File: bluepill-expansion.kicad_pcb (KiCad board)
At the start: 2 copper layers, 89.9 x 74.7 mm, 37 parts, among them J1 SENSE_A, J10 ENCODERS, J11 LS2, J12 I/O 3V3, J13 DIGITAL_PWR, J2 SENSE_B, J3 POWER_DC, J4 MOTDC1, J5 MOTDC2, J6 I2C, J7 UART, J8 CAN_BUS, J9 LS1, SW1 LS1, SW2 LS2, U1 BluePill_STM32F103C, U2 L298HN, U3 MCP2551-I-P

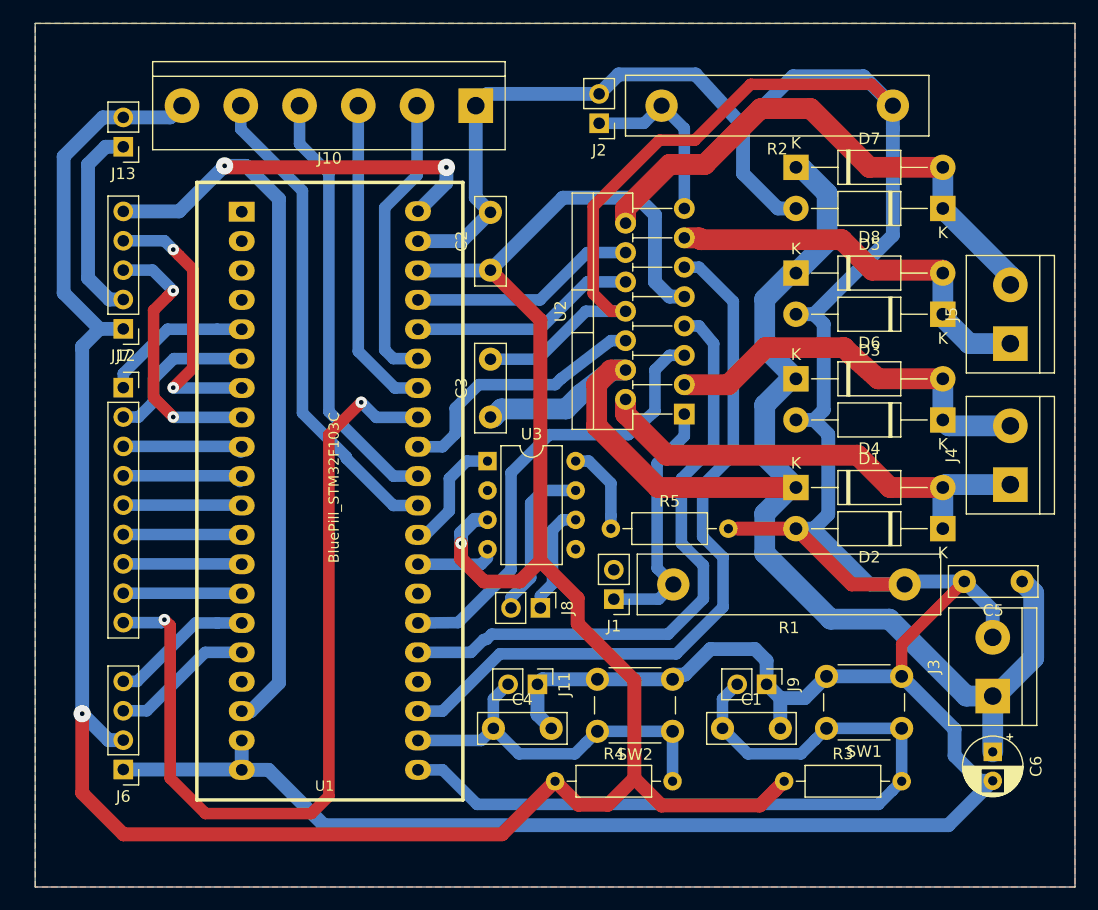
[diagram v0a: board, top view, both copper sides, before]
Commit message: update PCB
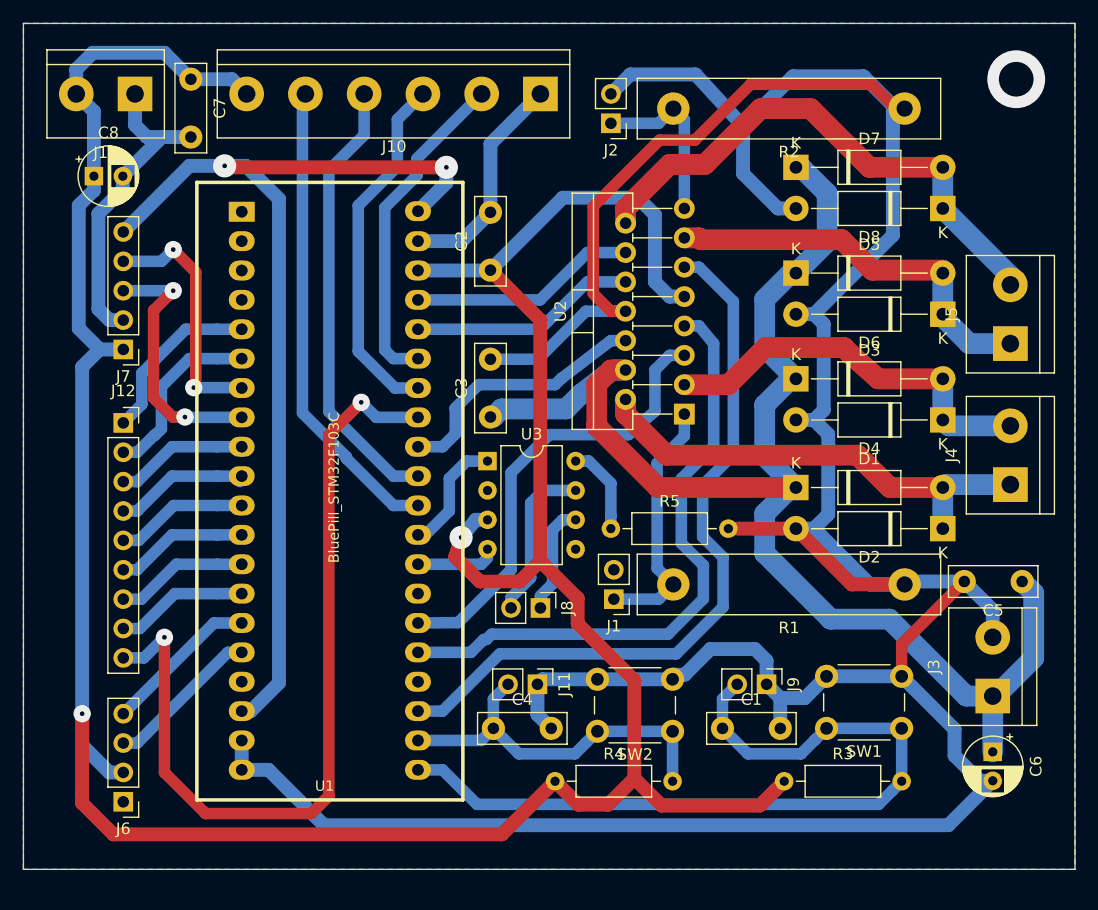
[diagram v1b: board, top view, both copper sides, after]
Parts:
- added C7: 0.1uF, Capacitor_THT:C_Disc_D7.5mm_W2.5mm_P5.00mm, F.Cu at (115.6, 57.7)
- added C8: 100uF, Capacitor_THT:CP_Radial_D5.0mm_P2.50mm, F.Cu at (107.2, 66.0)
- C6: value 10uF -> 470uF
- J13: footprint Connector_PinHeader_2.54mm:PinHeader_1x02_P2.54mm_Vertical -> TerminalBlock:TerminalBlock_bornier-2_P5.08mm
- moved J10 5.68 mm to (145.8, 58.9)
- moved J13 4.68 mm to (110.7, 58.9)
- moved J12 3.05 mm to (109.7, 87.4)
- moved J6 2.79 mm to (109.7, 120.1)
- moved J7 1.78 mm to (109.7, 81.0)
- moved R2 1.05 mm to (177.3, 60.2)
- moved J2 1.02 mm to (151.9, 61.5)
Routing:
- net +5V: track 238.7 -> 255.2 mm
- net GND: track 374.6 -> 364.9 mm
- net ENC2_Q: track 25.5 -> 28.8 mm
- net ENC2_D: track 27.7 -> 31.0 mm
- net UARTTX: track 24.6 -> 22.4 mm
- net /PA1: track 13.5 -> 15.7 mm
- net /PA0: track 13.0 -> 15.2 mm
- net /PB1: track 10.3 -> 11.5 mm
- net /PA7: track 10.3 -> 11.5 mm
- net /PB0: track 10.3 -> 11.5 mm
- net /PA6: track 10.6 -> 11.8 mm
- net /PA5: track 10.8 -> 12.1 mm
- net ENC1_Q: track 37.5 -> 38.7 mm
- net /PA4: track 10.8 -> 11.9 mm
- net SCL: track 12.3 -> 13.5 mm
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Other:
- board size 89.9 x 74.7 mm -> 90.9 x 73.2 mm
